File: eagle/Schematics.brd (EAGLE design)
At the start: 65 x 56 mm, 56 parts, among them IC1 ADE9000, K1 PIN20X2

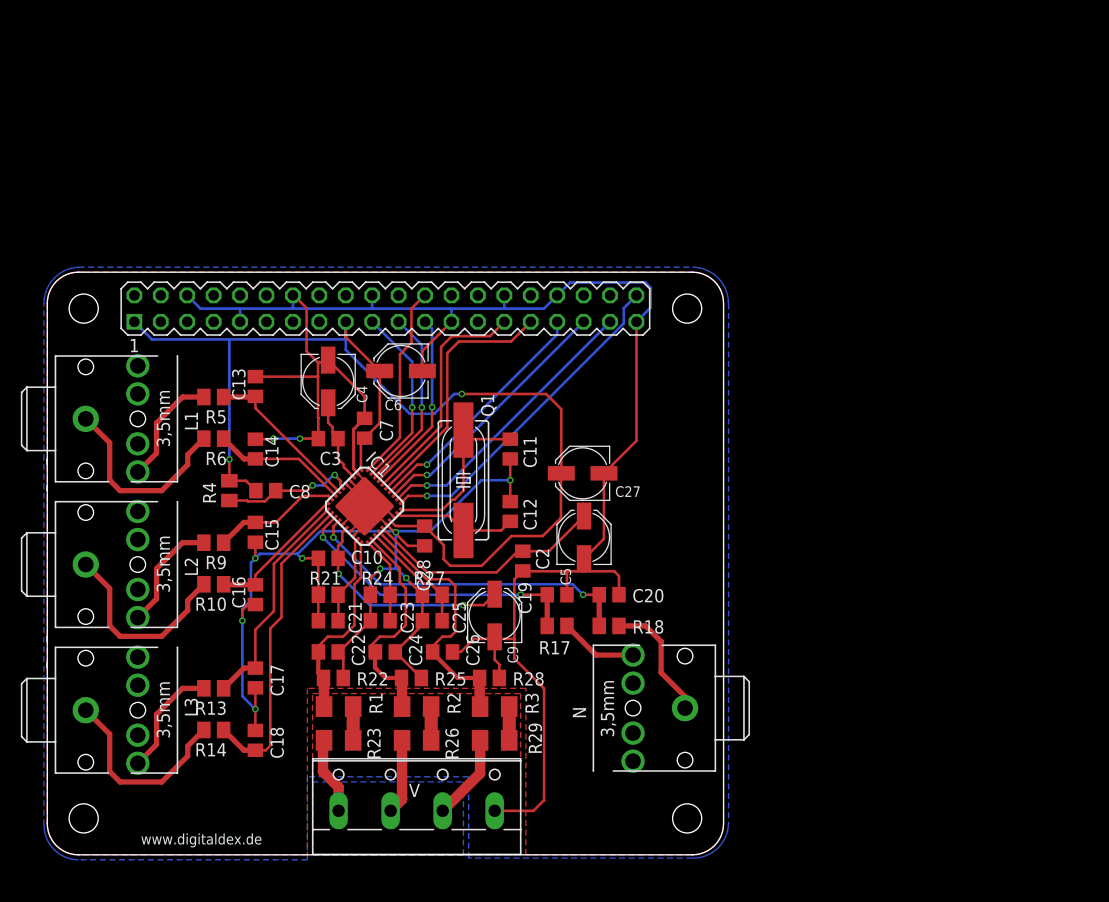
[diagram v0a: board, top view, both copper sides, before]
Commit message: Changes
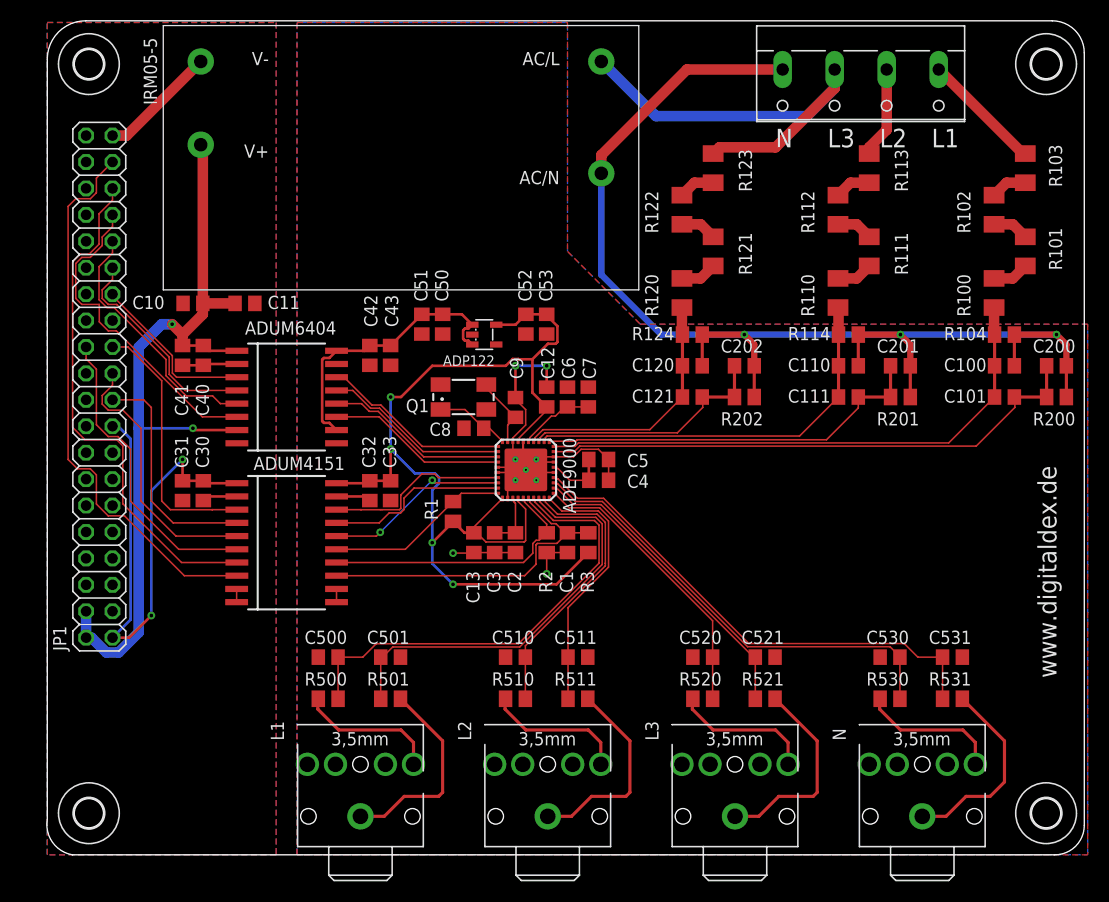
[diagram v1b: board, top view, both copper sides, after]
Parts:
- removed C14, C15, C16, C17, C18, C19, C20, C21, C22, C23, C24, C25, C26: 22nF, resistor:C0805
- removed C27: 10uF, resistor:PANASONIC_C
- removed C28: 0.1uF, resistor:C0805
- removed IC1: ADE9000, ADE9000:LFCSP40
- removed K1: PIN20X2, FLYFISH:PIN_20X2
- removed R10, R13, R14, R17, R18, R21, R22, R24, R25, R27, R28, R5, R6, R9: 1k, resistor:M0805
- removed R23, R26, R29: 500k, resistor:M1206
- removed R4: 10k, resistor:M0805
- removed V: (no value), con-wago-500:W237-4
- added ADE9000: ADE9000, ADE9000:LFCSP40
- added ADUM4151: ADUM4151, ADUM4151:SOIC20R
- added ADUM6404: ADUM6404, ADUM6404:SOIC16R
- added C1: 1uF, resistor:C0805
- added C100, C110, C120, C200, C201, C202, C500, C501, C510, C511, C520, C521, C530, C531: 22nF, resistor:C0805
- added C101, C111, C121: 51pF, resistor:C0805
- added C30, C32, C40, C42, C50, C52: 0.1uF, resistor:C0805
- added C31, C33, C41, C43, C51, C53: 10uF, resistor:C0805
- added IRM05-5: (no value), meanwell_irm_v6:IRM_05/10
- added JP1: (no value), adafruit:2X20
- added L: (no value), con-wago-500:W237-4
- added R100, R101, R102, R103, R110, R111, R112, R113, R120, R121, R122, R123: 200k, resistor:M1206
- added R104, R114, R124, R200, R201, R202, R500, R501, R510, R511, R520, R521, R530, R531: 1k, resistor:M0805
- added U$1, U$2, U$3, U$4: (no value), holes:2,8
- added U$5: ADP122AUJZ-3.3-R7, ADP122AUJZ-3.3-R7:TSOT23-5L
- C11: value 20pF -> 10uF
- C12: value 20pF -> 0.1uF
- C13: value 22nF -> 4.7uF
- C2: value 0.22uF -> 0.1uF
- C3: value 0.22uF -> 4.7uF
- C4: value 4.7uF -> 0.1uF; device resistor:PANASONIC_C -> resistor:C0805
- C5: device resistor:PANASONIC_C -> resistor:C0805
- C6: value 10uF -> 0.1uF; device resistor:PANASONIC_C -> resistor:C0805
- C7: value 0.1uF -> 4.7uF
- C8: value 1uF -> 18pF
- C9: value 4.7uF -> 18pF; device resistor:PANASONIC_C -> resistor:C0805
- Q1: device crystal:HC49UP -> crystal:CTS406
- R1, R2, R3: value 500k -> 10k; device resistor:M1206 -> resistor:M0805
- moved L3 66.3 mm to (66.0, 1.00), turned to 90 degrees
- moved L2 54.2 mm to (48.0, 1.00), turned to 90 degrees
- moved L1 50.2 mm to (30.0, 1.00), turned to 90 degrees
- moved C11 29.1 mm to (19.0, 53.0), turned to 0 degrees
- moved C10 27.7 mm to (14.0, 53.0)
- moved C4 27.7 mm to (53.0, 36.0), turned to 0 degrees
- moved C13 25.8 mm to (41.0, 30.0)
- moved N 23.9 mm to (84.0, 1.00), turned to 90 degrees
- moved R1 21.7 mm to (39.0, 33.0), turned to 270 degrees
- moved C7 21.7 mm to (52.0, 44.0)
- moved C8 20.9 mm to (41.0, 41.0), turned to 180 degrees
- moved R2 20.1 mm to (48.0, 30.0), turned to 90 degrees
- moved C9 20.1 mm to (45.0, 43.0)
- moved C3 18.9 mm to (43.0, 30.0), turned to 270 degrees
- moved R3 18.1 mm to (52.0, 30.0), turned to 270 degrees
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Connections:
- removed net +3V3: C27.+, C28.1, C6.+, C7.1, C8.1, IC1.1, IC1.27, K1.1, K1.17, R4.2
- removed net N$2: IC1.33, K1.35
- removed net N$24: IC1.39, K1.19
- removed net N$25: IC1.38, K1.21
- removed net N$26: IC1.37, K1.23
- removed net N$27: IC1.40, K1.24
- removed net N$5: C3.1, C4.+, IC1.3
- removed net N$6: C8.2, IC1.6, R4.1
- removed net N$7: C10.1, C9.+, IC1.16
- removed net N$8: C11.1, IC1.30, Q1.2
- removed net N$9: C12.2, IC1.29, Q1.1
- new net +3V3_ADE: ADE9000.1, ADE9000.27, ADE9000.4, ADUM4151.20, C12.1, C13.1, C32.1, C33.1, C52.1, C53.1, R1.2, R3.2, U$5.5
- new net +3V3_ISO: ADUM4151.1, C30.1, C31.1, JP1.1, JP1.17
- new net +5V_ADE: ADUM6404.10, ADUM6404.16, C42.1, C43.1, C50.1, C51.1, U$5.1, U$5.3
- new net +5V_ISO: ADUM6404.1, ADUM6404.7, C10.1, C11.1, C40.1, C41.1, IRM05-5.V+, JP1.2, JP1.4
- new net AGND: ADUM4151.10, ADUM4151.2, ADUM4151.9, ADUM6404.2, ADUM6404.8, C10.2, C11.2, C30.2, C31.2, C40.2, C41.2, IRM05-5.V-, JP1.14, JP1.20, JP1.25, JP1.30, JP1.34, JP1.39, JP1.6, JP1.9
- new net AVDDOUT: ADE9000.25, C6.1, C7.1
- new net CF1_ADE: ADE9000.33, ADUM6404.12
- new net CF1_ISO: ADUM6404.5, JP1.31
- new net CF2_ADE: ADE9000.34, ADUM6404.11
- new net CF2_ISO: ADUM6404.6, JP1.33
- new net CLKIN: ADE9000.29, C9.1, Q1.3
- new net CLKOUT: ADE9000.30, C8.1, Q1.1
- new net DVDDOUT: ADE9000.3, C2.1, C3.1
- new net IRQ0_ADE: ADE9000.31, ADUM6404.14
- new net IRQ0_ISO: ADUM6404.3, JP1.27
- new net IRQ1_ADE: ADE9000.32, ADUM6404.13
- new net IRQ1_ISO: ADUM6404.4, JP1.29
- new net MISO_ADE: ADE9000.38, ADUM4151.16
- new net MISO_ISO: ADUM4151.5, JP1.21
- new net MOSI_ADE: ADE9000.39, ADUM4151.17
- new net MOSI_ISO: ADUM4151.4, JP1.19
- new net PM1_ADE: ADE9000.5, ADUM4151.14, R2.2
- new net PM1_ISO: ADUM4151.7, JP1.35
- new net REF: ADE9000.16, C4.1, C5.1
- new net RESET_ADE: ADE9000.6, ADUM4151.13, C1.1, R3.1
- new net RESET_ISO: ADUM4151.8, JP1.37
- new net SCLK_ADE: ADE9000.37, ADUM4151.18
- new net SCLK_ISO: ADUM4151.3, JP1.23
- new net SS_ADE: ADE9000.40, ADUM4151.15, R1.1
- new net SS_ISO: ADUM4151.6, JP1.24
- net GND: now also ADE9000.15, ADE9000.17, ADE9000.18, ADE9000.2, ADE9000.26, ADE9000.28, ADE9000.35, ADE9000.36, ADE9000.GND, ADUM4151.11, ADUM4151.12, ADUM4151.19, ADUM6404.15, ADUM6404.9, C1.2, C100.1, C110.1, C12.2, C120.1, C13.2, C200.1, C201.1, C202.1, C32.2, C33.2, C4.2, C42.2, C43.2, C5.2, C50.2, C500.1, C501.2, C51.2, C510.1, C511.2, C52.2, C520.1, C521.2, C53.2, C530.1, C531.2, C6.2, C8.2, C9.2, IRM05-5.AC/N, L.4, R104.2, R114.2, R124.2, R2.1, R200.2, R201.2, R202.2, U$5.2, U$5.4; no longer C10.2, C11.2, C12.1, C13.1, C14.2, C15.1, C16.2, C17.1, C18.2, C19.1, C20.2, C21.1, C22.1, C23.1, C24.1, C25.1, C26.1, C27.-, C28.2, C4.-, C5.-, C6.-, C9.-, IC1.15, IC1.17, IC1.18, IC1.2, IC1.26, IC1.28, IC1.4, IC1.5, IC1.GND, K1.14, K1.20, K1.25, K1.30, K1.34, K1.39, K1.6, K1.9, R21.2, R22.2, R24.2, R25.2, R27.2, R28.2, V.4
- net IAN: now also ADE9000.8, C501.1, R501.1; no longer C14.1, IC1.8, R6.1
- net IAP: now also ADE9000.7, C500.2, R500.1; no longer C13.2, IC1.7, R5.1
- net IBN: now also ADE9000.10, C511.1, R511.1; no longer C16.1, IC1.10, R10.1
- net IBP: now also ADE9000.9, C510.2, R510.1; no longer C15.2, IC1.9, R9.1
- net ICN: now also ADE9000.12, C521.1, R521.1; no longer C18.1, IC1.12, R14.1
- net ICP: now also ADE9000.11, C520.2, R520.1; no longer C17.2, IC1.11, R13.1
- net INN: now also ADE9000.14, C531.1, R531.1; no longer C20.1, IC1.14, R18.1
- net INP: now also ADE9000.13, C530.2, R530.1; no longer C19.2, IC1.13, R17.1
- net N$1: now also R121.2, R122.1; no longer IC1.32, K1.37
- net N$10: now also R500.2; no longer R5.2
- net N$11: now also R501.2; no longer R6.2
- net N$12: now also R510.2; no longer R9.2
- net N$13: now also R511.2; no longer R10.2
- net N$14: now also R520.2; no longer R13.2
- net N$15: now also R521.2; no longer R14.2
- net N$16: now also R530.2; no longer R17.2
- net N$17: now also R531.2; no longer R18.2
- net N$18: now also R101.2, R102.1; no longer R23.2, V.1
- net N$19: now also R111.2, R112.1; no longer R26.2, V.2
- net N$20: now also R112.2, R113.1; no longer R29.2, V.3
- net N$21: now also R122.2, R123.1; no longer IC1.35, K1.31
- net N$22: now also L.2, R113.2; no longer IC1.36, K1.29
- net N$23: now also IRM05-5.AC/L, L.3, R123.2; no longer IC1.31, K1.40
- net N$29: now also R110.2, R111.1; no longer R2.2, R26.1
- net N$3: now also R102.2, R103.1; no longer IC1.34, K1.33
- net N$30: now also R100.2, R101.1; no longer R1.2, R23.1
- net N$31: now also R120.2, R121.1; no longer R29.1, R3.2
- net N$4: now also L.1, R103.2; no longer C2.1, C5.+, IC1.25
- net VAN: now also ADE9000.19, C101.1, C200.2, R200.1; no longer C21.2, IC1.19, R21.1
- net VAP: now also ADE9000.20, C100.2, C101.2, R100.1, R104.1; no longer C22.2, IC1.20, R1.1, R22.1
- net VBN: now also ADE9000.21, C111.1, C201.2, R201.1; no longer C23.2, IC1.21, R24.1
- net VBP: now also ADE9000.22, C110.2, C111.2, R110.1, R114.1; no longer C24.2, IC1.22, R2.1, R25.1
- net VCN: now also ADE9000.23, C121.1, C202.2, R202.1; no longer C25.2, IC1.23, R27.1
- net VCP: now also ADE9000.24, C120.2, C121.2, R120.1, R124.1; no longer C26.2, IC1.24, R28.1, R3.1
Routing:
- net GND: track 307.2 -> 181.7 mm, vias 10 -> 11
- net +3V3: track 114.2 -> 0.00 mm, vias 2 -> 0
- net +3V3_ADE: track 0.00 -> 100.5 mm, vias 0 -> 4
- net +5V_ISO: track 0.00 -> 80.2 mm, vias 0 -> 2
- net RESET_ISO: track 0.00 -> 53.7 mm
- net +3V3_ISO: track 0.00 -> 50.3 mm, vias 0 -> 2
- net PM1_ISO: track 0.00 -> 49.5 mm
- net VAN: track 9.56 -> 53.1 mm
- net VAP: track 19.4 -> 52.9 mm
- net RESET_ADE: track 0.00 -> 32.3 mm
- net CF2_ISO: track 0.00 -> 31.2 mm
- net VBN: track 8.33 -> 38.2 mm
- net SS_ISO: track 0.00 -> 29.3 mm
- net IAP: track 15.5 -> 44.0 mm
- net +5V_ADE: track 0.00 -> 28.1 mm
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- added copper zone on layer 1, net AGND
- added copper zone on layer 16, net AGND
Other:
- board size 65 x 56 mm -> 99.7 x 80.2 mm
- board text added: "ADP122"
- board text added: "ADUM6404"
- board text added: "L1"
- board text added: "L2"
- board text added: "L3"
- board text added: "N"
